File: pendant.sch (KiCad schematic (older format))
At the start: 3 parts, among them J1 AudioJack4_Ground, J2 AudioJack4_Ground, U1 BlackPillSymple

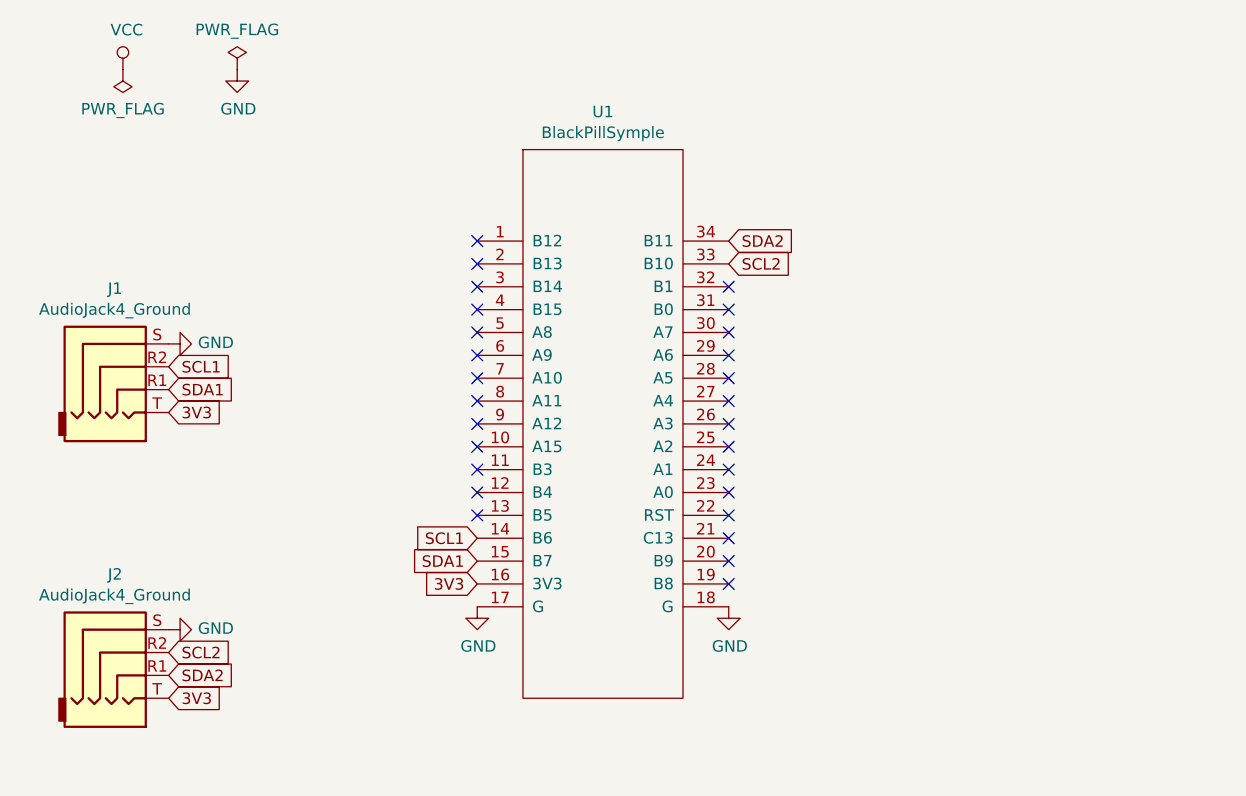
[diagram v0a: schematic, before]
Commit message: Update schematics for beta
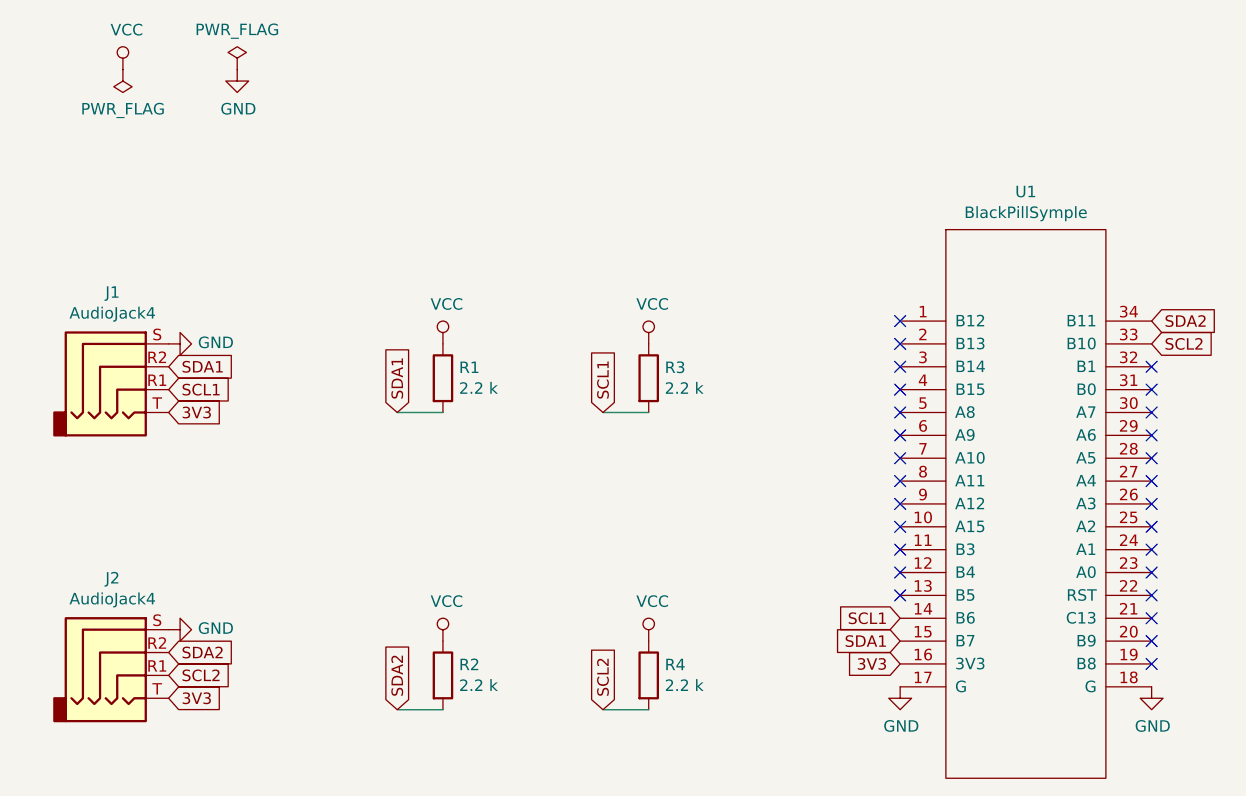
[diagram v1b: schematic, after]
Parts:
- removed J1, J2: AudioJack4_Ground, library:TRRS_SMD_PJ320, symbol Connector:AudioJack4_Ground
- added J1, J2: AudioJack4, library:TRRS_SMD_PJ320, symbol Connector:AudioJack4
- added R1, R2, R3, R4: 2.2 k, Resistor_SMD:R_0603_1608Metric, symbol Device:R
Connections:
- net 3V3: now also J1.T, J2.T
- net GND: now also J1.S, J2.S
- net SCL1: now also J1.R1, R3.2
- net SCL2: now also J2.R1, R4.2
- net SDA1: now also J1.R2, R1.2
- net SDA2: now also J2.R2, R2.2
- net VCC: now also R1.1, R2.1, R3.1, R4.1
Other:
- moved on the sheet: U1
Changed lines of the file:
@@
 EESchema Schematic File Version 4
+LIBS:pendant-cache
 EELAYER 26 0
 EELAYER END
@@
 L BlackPill:BlackPillSymple U1
 U 1 1 5BC1C845
-P 3600 2850
-F 0 "U1" H 3600 4215 50  0000 C CNN
-F 1 "BlackPillSymple" H 3600 4124 50  0000 C CNN
-F 2 "library:BlackPillSimple" H 3600 700 50  0001 C CNN
-F 3 "" H 3600 700 50  0001 C CNN
-	1    3600 2850
-	1    0    0    -1
-$EndComp
-NoConn ~ 4150 2250
-NoConn ~ 4150 2350
-NoConn ~ 4150 2450
-NoConn ~ 4150 2550
-NoConn ~ 4150 2650
-NoConn ~ 4150 2750
-NoConn ~ 4150 2850
-NoConn ~ 4150 2950
-NoConn ~ 4150 3050
-NoConn ~ 4150 3150
-NoConn ~ 4150 3250
-NoConn ~ 4150 3350
-NoConn ~ 4150 3450
-NoConn ~ 4150 3550
-NoConn ~ 3050 3250
-NoConn ~ 3050 3150
-NoConn ~ 3050 3050
-NoConn ~ 3050 2950
-NoConn ~ 3050 2850
-NoConn ~ 3050 2750
-NoConn ~ 3050 2650
-NoConn ~ 3050 2550
-NoConn ~ 3050 2450
-NoConn ~ 3050 2350
-NoConn ~ 3050 2250
-NoConn ~ 3050 2150
-NoConn ~ 3050 2050
+P 5450 3200
+F 0 "U1" H 5450 4565 50  0000 C CNN
+F 1 "BlackPillSymple" H 5450 4474 50  0000 C CNN
+F 2 "library:BlackPillSimple" H 5450 1050 50  0001 C CNN
+F 3 "" H 5450 1050 50  0001 C CNN
+	1    5450 3200
+	1    0    0    -1
+$EndComp
+NoConn ~ 6000 2600
+NoConn ~ 6000 2700
+NoConn ~ 6000 2800
+NoConn ~ 6000 2900
+NoConn ~ 6000 3000
+NoConn ~ 6000 3100
+NoConn ~ 6000 3200
+NoConn ~ 6000 3300
+NoConn ~ 6000 3400
+NoConn ~ 6000 3500
+NoConn ~ 6000 3600
+NoConn ~ 6000 3700
+NoConn ~ 6000 3800
+NoConn ~ 6000 3900
+NoConn ~ 4900 3600
+NoConn ~ 4900 3500
+NoConn ~ 4900 3400
+NoConn ~ 4900 3300
+NoConn ~ 4900 3200
+NoConn ~ 4900 3100
+NoConn ~ 4900 3000
+NoConn ~ 4900 2900
+NoConn ~ 4900 2800
+NoConn ~ 4900 2700
+NoConn ~ 4900 2600
+NoConn ~ 4900 2500
+NoConn ~ 4900 2400
 $Comp
 L power:VCC #PWR01
@@
 L power:GND #PWR06
 U 1 1 5BC1CC6F
-P 4150 3650
-F 0 "#PWR06" H 4150 3400 50  0001 C CNN
-F 1 "GND" H 4155 3477 50  0000 C CNN
-F 2 "" H 4150 3650 50  0001 C CNN
-F 3 "" H 4150 3650 50  0001 C CNN
-	1    4150 3650
+P 6000 4000
+F 0 "#PWR06" H 6000 3750 50  0001 C CNN
+F 1 "GND" H 6005 3827 50  0000 C CNN
+F 2 "" H 6000 4000 50  0001 C CNN
+F 3 "" H 6000 4000 50  0001 C CNN
+	1    6000 4000
 	1    0    0    -1
 $EndComp
@@
 L power:GND #PWR05
 U 1 1 5BC1CC94
-P 3050 3650
-F 0 "#PWR05" H 3050 3400 50  0001 C CNN
-F 1 "GND" H 3055 3477 50  0000 C CNN
-F 2 "" H 3050 3650 50  0001 C CNN
-F 3 "" H 3050 3650 50  0001 C CNN
-	1    3050 3650
-	1    0    0    -1
-$EndComp
-Text GLabel 4150 2050 2    50   Input ~ 0
+P 4900 4000
+F 0 "#PWR05" H 4900 3750 50  0001 C CNN
+F 1 "GND" H 4905 3827 50  0000 C CNN
+F 2 "" H 4900 4000 50  0001 C CNN
+F 3 "" H 4900 4000 50  0001 C CNN
+	1    4900 4000
+	1    0    0    -1
+$EndComp
+Text GLabel 6000 2400 2    50   Input ~ 0
 SDA2
-Text GLabel 4150 2150 2    50   Input ~ 0
+Text GLabel 6000 2500 2    50   Input ~ 0
 SCL2
-Text GLabel 3050 3350 0    50   Input ~ 0
+Text GLabel 4900 3700 0    50   Input ~ 0
 SCL1
-Text GLabel 3050 3450 0    50   Input ~ 0
+Text GLabel 4900 3800 0    50   Input ~ 0
 SDA1
-Text GLabel 3050 3550 0    50   Input ~ 0
+Text GLabel 4900 3900 0    50   Input ~ 0
 3V3
-$Comp
-L Connector:AudioJack4_Ground J1
-U 1 1 5BC1CE18
-P 1500 2600
-F 0 "J1" H 1466 2942 50  0000 C CNN
-F 1 "AudioJack4_Ground" H 1466 2851 50  0000 C CNN
-F 2 "library:TRRS_SMD_PJ320" H 1500 2600 50  0001 C CNN
-F 3 "~" H 1500 2600 50  0001 C CNN
-	1    1500 2600
-	1    0    0    -1
-$EndComp
-$Comp
-L Connector:AudioJack4_Ground J2
-U 1 1 5BC1CEFE
-P 1500 3850
-F 0 "J2" H 1466 4192 50  0000 C CNN
-F 1 "AudioJack4_Ground" H 1466 4101 50  0000 C CNN
-F 2 "library:TRRS_SMD_PJ320" H 1500 3850 50  0001 C CNN
-F 3 "~" H 1500 3850 50  0001 C CNN
-	1    1500 3850
-	1    0    0    -1
-$EndComp
 Text GLabel 1700 2800 2    50   Input ~ 0
 3V3
@@
 	0    -1   -1   0
 $EndComp
+Text GLabel 1700 2600 2    50   Input ~ 0
+SDA1
 Text GLabel 1700 2700 2    50   Input ~ 0
-SDA1
-Text GLabel 1700 2600 2    50   Input ~ 0
 SCL1
 Text GLabel 1700 4050 2    50   Input ~ 0
 3V3
+Text GLabel 1700 3850 2    50   Input ~ 0
+SDA2
 Text GLabel 1700 3950 2    50   Input ~ 0
-SDA2
-Text GLabel 1700 3850 2    50   Input ~ 0
 SCL2
 $Comp
@@
 	0    -1   -1   0
 $EndComp
+$Comp
+L Connector:AudioJack4 J1
+U 1 1 5C162EB1
+P 1500 2600
+F 0 "J1" H 1455 2925 50  0000 C CNN
+F 1 "AudioJack4" H 1455 2834 50  0000 C CNN
+F 2 "library:TRRS_SMD_PJ320" H 1500 2600 50  0001 C CNN
+F 3 "~" H 1500 2600 50  0001 C CNN
+	1    1500 2600
+	1    0    0    -1
+$EndComp
+$Comp
+L Connector:AudioJack4 J2
+U 1 1 5C162F8A
+P 1500 3850
+F 0 "J2" H 1455 4175 50  0000 C CNN
+F 1 "AudioJack4" H 1455 4084 50  0000 C CNN
+F 2 "library:TRRS_SMD_PJ320" H 1500 3850 50  0001 C CNN
+F 3 "~" H 1500 3850 50  0001 C CNN
+	1    1500 3850
+	1    0    0    -1
+$EndComp
+$Comp
+L power:VCC #PWR09
+U 1 1 5C1630AE
+P 3800 2500
+F 0 "#PWR09" H 3800 2350 50  0001 C CNN
+F 1 "VCC" H 3817 2673 50  0000 C CNN
+F 2 "" H 3800 2500 50  0001 C CNN
+F 3 "" H 3800 2500 50  0001 C CNN
+	1    3800 2500
+	1    0    0    -1
+$EndComp
+$Comp
+L Device:R R3
+U 1 1 5C1630EE
+P 3800 2650
+F 0 "R3" H 3870 2696 50  0000 L CNN
+F 1 "2.2 k" H 3870 2605 50  0000 L CNN
+F 2 "Resistor_SMD:R_0603_1608Metric" V 3730 2650 50  0001 C CNN
+F 3 "~" H 3800 2650 50  0001 C CNN
+	1    3800 2650
+	1    0    0    -1
+$EndComp
+Wire Wire Line
+	3800 2800 3600 2800
+Text GLabel 3600 2800 1    50   Input ~ 0
+SCL1
+$Comp
+L power:VCC #PWR07
+U 1 1 5C1631FC
+P 2900 2500
+F 0 "#PWR07" H 2900 2350 50  0001 C CNN
+F 1 "VCC" H 2917 2673 50  0000 C CNN
+F 2 "" H 2900 2500 50  0001 C CNN
+F 3 "" H 2900 2500 50  0001 C CNN
+	1    2900 2500
+	1    0    0    -1
+$EndComp
+$Comp
+L Device:R R1
+U 1 1 5C163202
+P 2900 2650
+F 0 "R1" H 2970 2696 50  0000 L CNN
+F 1 "2.2 k" H 2970 2605 50  0000 L CNN
+F 2 "Resistor_SMD:R_0603_1608Metric" V 2830 2650 50  0001 C CNN
+F 3 "~" H 2900 2650 50  0001 C CNN
+	1    2900 2650
+	1    0    0    -1
+$EndComp
+Wire Wire Line
+	2900 2800 2700 2800
+Text GLabel 2700 2800 1    50   Input ~ 0
+SDA1
+$Comp
+L power:VCC #PWR010
+U 1 1 5C1632C1
+P 3800 3800
+F 0 "#PWR010" H 3800 3650 50  0001 C CNN
+F 1 "VCC" H 3817 3973 50  0000 C CNN
+F 2 "" H 3800 3800 50  0001 C CNN
+F 3 "" H 3800 3800 50  0001 C CNN
+	1    3800 3800
+	1    0    0    -1
+$EndComp
+$Comp
+L Device:R R4
+U 1 1 5C1632C7
+P 3800 3950
+F 0 "R4" H 3870 3996 50  0000 L CNN
+F 1 "2.2 k" H 3870 3905 50  0000 L CNN
+F 2 "Resistor_SMD:R_0603_1608Metric" V 3730 3950 50  0001 C CNN
+F 3 "~" H 3800 3950 50  0001 C CNN
+	1    3800 3950
+	1    0    0    -1
+$EndComp
+Wire Wire Line
+	3800 4100 3600 4100
+Text GLabel 3600 4100 1    50   Input ~ 0
+SCL2
+$Comp
+L power:VCC #PWR08
+U 1 1 5C1632CF
+P 2900 3800
+F 0 "#PWR08" H 2900 3650 50  0001 C CNN
+F 1 "VCC" H 2917 3973 50  0000 C CNN
+F 2 "" H 2900 3800 50  0001 C CNN
+F 3 "" H 2900 3800 50  0001 C CNN
+	1    2900 3800
+	1    0    0    -1
+$EndComp
+$Comp
+L Device:R R2
+U 1 1 5C1632D5
+P 2900 3950
+F 0 "R2" H 2970 3996 50  0000 L CNN
+F 1 "2.2 k" H 2970 3905 50  0000 L CNN
+F 2 "Resistor_SMD:R_0603_1608Metric" V 2830 3950 50  0001 C CNN
+F 3 "~" H 2900 3950 50  0001 C CNN
+	1    2900 3950
+	1    0    0    -1
+$EndComp
+Wire Wire Line
+	2900 4100 2700 4100
+Text GLabel 2700 4100 1    50   Input ~ 0
+SDA2
 $EndSCHEMATC
